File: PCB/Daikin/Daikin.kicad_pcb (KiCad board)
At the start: 2 copper layers, 15.2 x 20 mm, 22 parts, among them J1 1x5, J2 Prog, Q3 PMF250XNEX, U1 ESP32-PICO-MINI-02, U2 LMR16006YDDCR

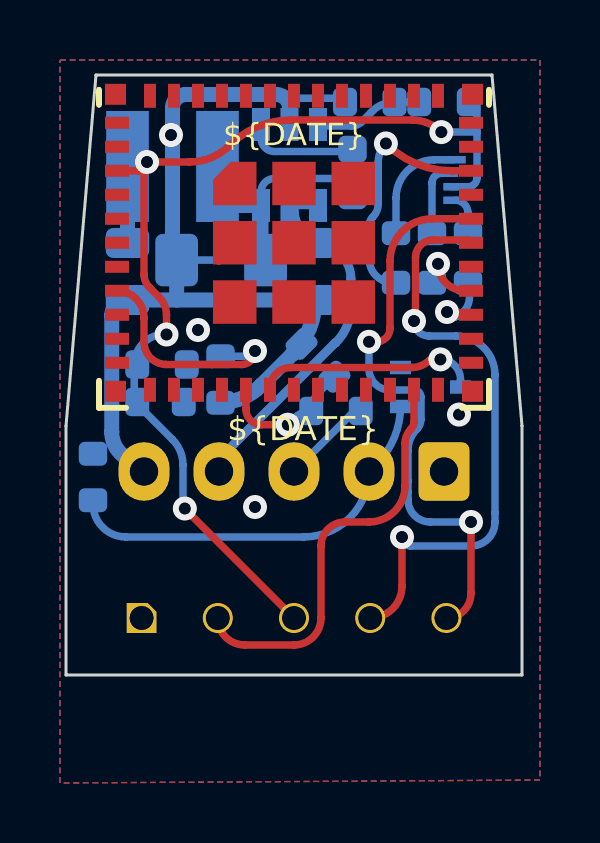
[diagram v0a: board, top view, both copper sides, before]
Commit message: Revised for production
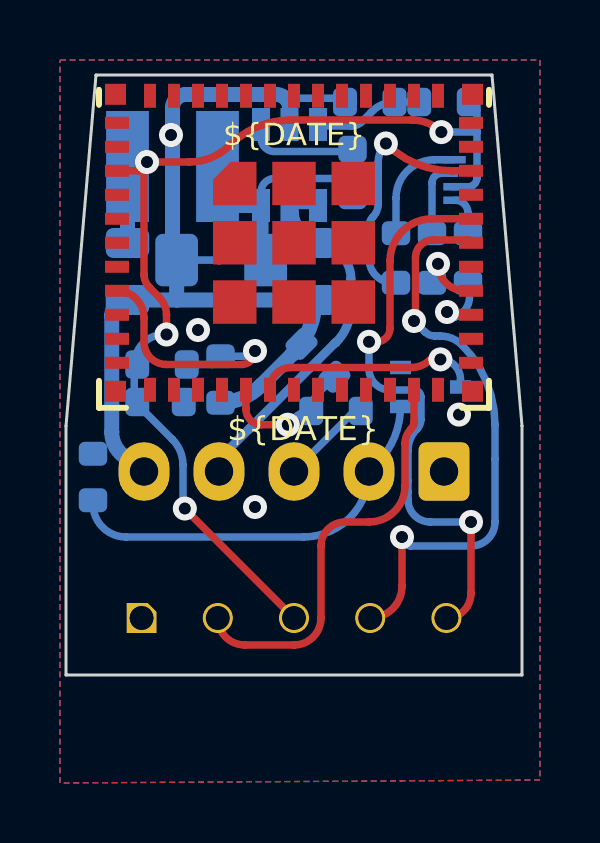
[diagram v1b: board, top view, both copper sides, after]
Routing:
- net Net-(J2-Pad4): track 20.0 -> 19.5 mm
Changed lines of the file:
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@@
     )
   )
-  (property "DATE" "2023-03-31")
+  (property "DATE" "2023-04-08")
   (net 0 "")
   (net 1 "GND")
@@
     (descr "Capacitor SMD 0603 (1608 Metric), square (rectangular) end terminal, IPC_7351 nominal, (Body size source: IPC-SM-782 page 76, https://www.pcb-3d.com/wordpress/wp-content/uploads/ipc-sm-782a_amendment_1_and_2.pdf), generated with kicad-footprint-generator")
     (tags "capacitor")
+    (property "JLCPCB Rotation Offset" "90")
     (property "Manufacturer" "")
     (property "Note" "")
@@
   (arc (start 105.80675 44) (mid 105.872688 44.027312) (end 105.9 44.09325) (width 0.25) (layer "F.Cu") (net 36))
   (arc (start 104.05 44.585704) (mid 104.221549 44.171549) (end 104.635704 44) (width 0.25) (layer "F.Cu") (net 36))
+  (segment (start 104.7 47.2) (end 104.875736 47.2) (width 0.25) (layer "B.Cu") (net 36))
+  (segment (start 106.7 51.3) (end 106.7 50.155634) (width 0.25) (layer "B.Cu") (net 36))
   (segment (start 105.9 54.2) (end 103.9 54.2) (width 0.25) (layer "B.Cu") (net 36))
-  (segment (start 106.7 53.1) (end 106.7 48.5) (width 0.25) (layer "B.Cu") (net 36))
-  (segment (start 104.5 47.2) (end 105.4 47.2) (width 0.25) (layer "B.Cu") (net 36))
-  (segment (start 106.7 53.1) (end 106.7 53.4) (width 0.25) (layer "B.Cu") (net 36))
-  (arc (start 104 46.7) (mid 104.146447 47.053553) (end 104.5 47.2) (width 0.25) (layer "B.Cu") (net 36))
-  (arc (start 106.7 48.5) (mid 106.319239 47.580761) (end 105.4 47.2) (width 0.25) (layer "B.Cu") (net 36))
+  (segment (start 104 46.7) (end 104.358578 47.058578) (width 0.25) (layer "B.Cu") (net 36))
+  (segment (start 106.7 53.4) (end 106.7 51.3) (width 0.25) (layer "B.Cu") (net 36))
+  (arc (start 106.7 50.155634) (mid 106.414119 48.718415) (end 105.6 47.5) (width 0.25) (layer "B.Cu") (net 36))
+  (arc (start 104.875736 47.2) (mid 105.267704 47.277968) (end 105.6 47.5) (width 0.25) (layer "B.Cu") (net 36))
   (arc (start 106.7 53.4) (mid 106.465685 53.965685) (end 105.9 54.2) (width 0.25) (layer "B.Cu") (net 36))
+  (arc (start 104.358578 47.058578) (mid 104.515224 47.163245) (end 104.7 47.2) (width 0.25) (layer "B.Cu") (net 36))
   (arc (start 103.9 54.2) (mid 103.687868 54.112132) (end 103.6 53.9) (width 0.25) (layer "B.Cu") (net 36))
   (segment (start 103.2 46.94325) (end 103.2 44.7) (width 0.25) (layer "F.Cu") (net 37))
